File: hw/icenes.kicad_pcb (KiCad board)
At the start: 6 copper layers, 201 parts, among them J1 USB_B_Micro, J2 Barrel_Jack_Switch, J3 Conn_02x11_Odd_Even, J4 Conn_02x31_Odd_Even, J5 Conn_02x31_Odd_Even, J6 NES-Connector-72pin, U1 TPS62050, U10 74ALVC164245, U11 74ALVC164245, U12 74ALVC164245, U13 74ALVC164245, U2 TPS62050, U3 TPS62056, U4 iCE40HX8K-CT256, U5 93LC56C-I_SN, U6 FT2232H, U7 AT25SF041-SSHD, U8 SN74LVC1404, U9 SN74LVC1404, X1 DSC1001DI2-012.0000, Y1 21.47727MHz, Y2 26.601712MHz

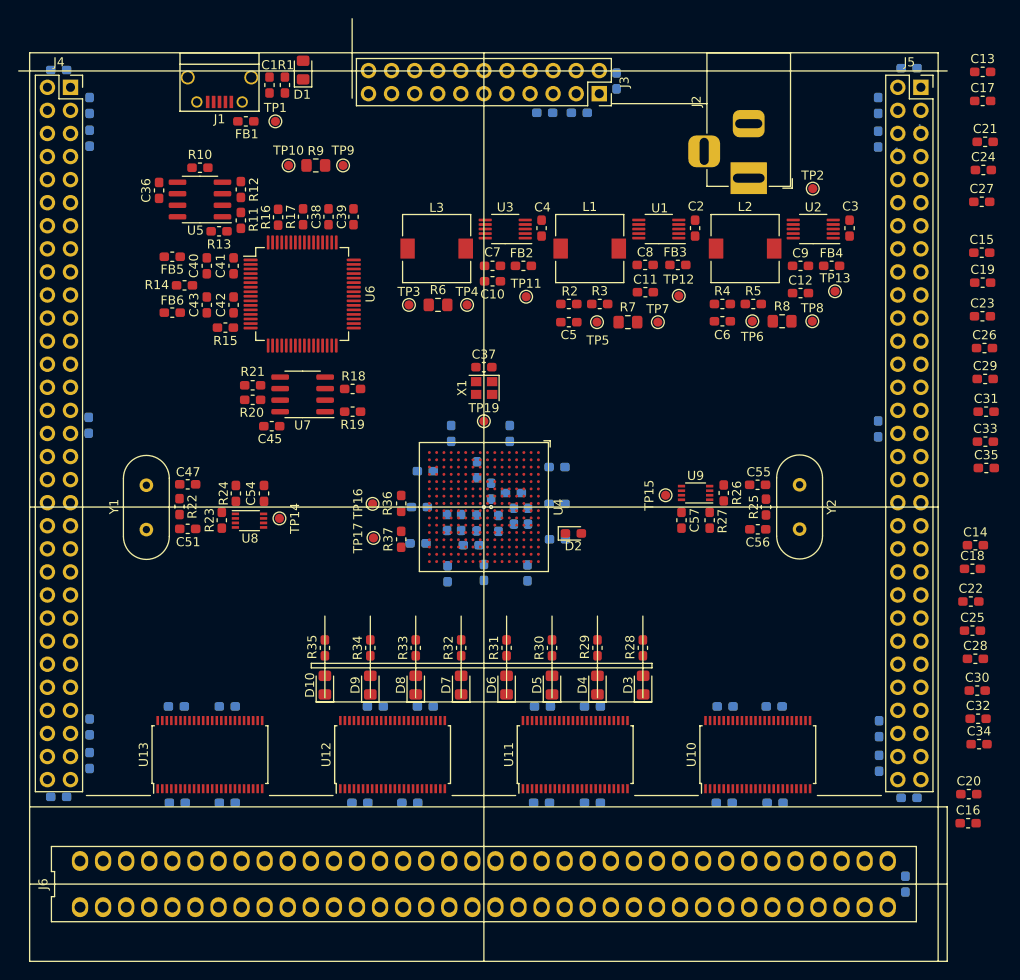
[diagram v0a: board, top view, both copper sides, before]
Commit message: Layout.
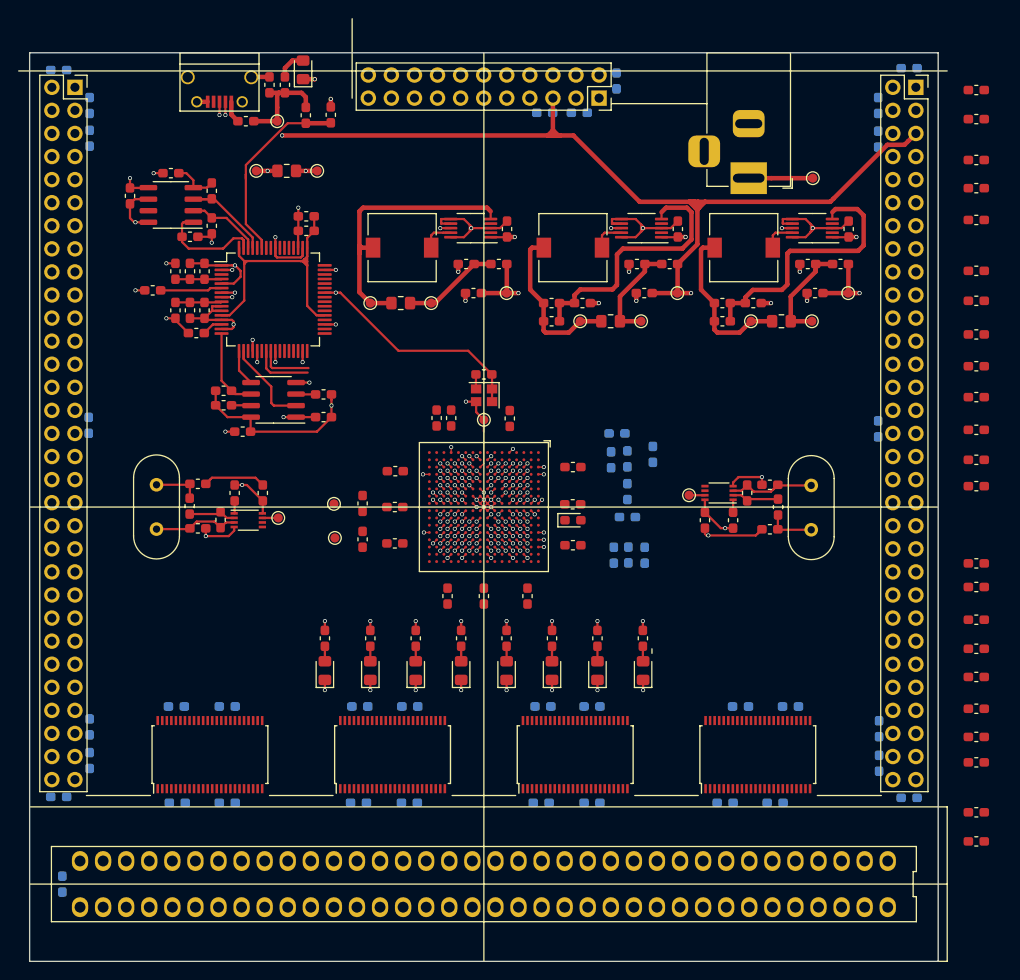
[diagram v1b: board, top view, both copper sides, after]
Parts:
- C48, C49, C52, C59, C61, C63, C65, C68, C75, C79, C82, C87: moved to F.Cu
- moved C106 92.8 mm to (53.6, 141.5), turned to 90 degrees
- moved C103 40.2 mm to (132.1, 132.6)
- moved C100 40.2 mm to (133.8, 122.0)
- moved C105 40.2 mm to (126.5, 132.6)
- moved C98 40.2 mm to (128.2, 122.0)
- moved U12 40.2 mm to (130.2, 127.2)
- moved C95 20.2 mm to (111.9, 132.6)
- moved C96 20.2 mm to (91.8, 132.6)
- moved C97 20.2 mm to (106.3, 132.6)
- moved C94 20.1 mm to (86.2, 132.6)
- moved C91 20.1 mm to (86.3, 122.0)
- moved C93 20.1 mm to (91.8, 122.0)
- moved U10 20.1 mm to (110.0, 127.2)
- moved U11 20.1 mm to (90.0, 127.2)
- moved C92 20.0 mm to (106.5, 122.0)
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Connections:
- net USB_DM renamed USB_D_N
- net USB_DP renamed USB_D_P
- C60 pad 1: +5V -> +1V2
- C64 pad 1: +1V2 -> +5V
- C66 pad 1: +5V -> +1V2
- C67 pad 2: +5V -> +1V2
- C77 pad 1: +1V2 -> +5V
- C78 pad 2: +1V2 -> +5V
- C80 pad 1: +5V -> +1V2
- C81 pad 2: +5V -> +1V2
- C88 pad 1: +1V2 -> +5V
- C89 pad 2: +1V2 -> +5V
- J3 pad 1: +1V2 -> +5V
- J3 pad 5: +5V -> +1V2
- J4 pad 1: +1V2 -> +5V
- J4 pad 5: +5V -> +1V2
- J4 pad 57: +5V -> +1V2
- J4 pad 61: +1V2 -> +5V
- J5 pad 1: +1V2 -> +5V
- J5 pad 5: +5V -> +1V2
- J5 pad 57: +5V -> +1V2
- J5 pad 61: +1V2 -> +5V
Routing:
- net GND: track 0.00 -> 137.4 mm, vias 2 -> 47
- net +1V2: track 0.04 -> 107.1 mm, vias 0 -> 10
- net +3V3: track 0.00 -> 71.7 mm, vias 0 -> 22
- net +3V3_FTDI: track 0.00 -> 49.9 mm, vias 0 -> 10
- net ICE_CLK_12MHZ: track 0.00 -> 41.7 mm, vias 0 -> 2
- net +1V8_FTDI: track 0.00 -> 31.8 mm
- net Net-(L3-Pad2): track 0.00 -> 30.8 mm
- net Net-(C5-Pad2): track 0.00 -> 29.5 mm
- net Net-(C6-Pad2): track 0.00 -> 29.4 mm
- net USB_D_N: track 0.00 -> 27.5 mm, vias 0 -> 2
- net USB_D_P: track 0.00 -> 27.5 mm, vias 0 -> 2
- net Net-(R16-Pad2): track 0.00 -> 21.6 mm
- net /Vin(+5V-+10V): track 0.00 -> 18.8 mm, vias 0 -> 6
- net Net-(C6-Pad1): track 0.00 -> 18.1 mm
- net Net-(C5-Pad1): track 0.00 -> 18.1 mm
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- added copper zone on In4.Cu, net +1V2
- added copper zone on In4.Cu, net +3V3
- added copper zone on In4.Cu, net +3V3_FTDI
- added copper zone on In4.Cu, net +5V
- added copper zone on In4.Cu, net /Vin(+5V-+10V)
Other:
- board outline added: 100 x 100 mm
- net class Default: clearance 0.15 -> 0.127
- rule trace_clearance: 0.15 -> 0.127
